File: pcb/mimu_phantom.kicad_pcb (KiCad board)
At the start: 2 copper layers, 50 x 27 mm, 35 parts, among them J1 OPT, SW1 SW_Push, SW2 SW_SPDT, U1 AQY211EH, U2 ATTINY88AU, U3 MCP16331CH, U4 H11F1M

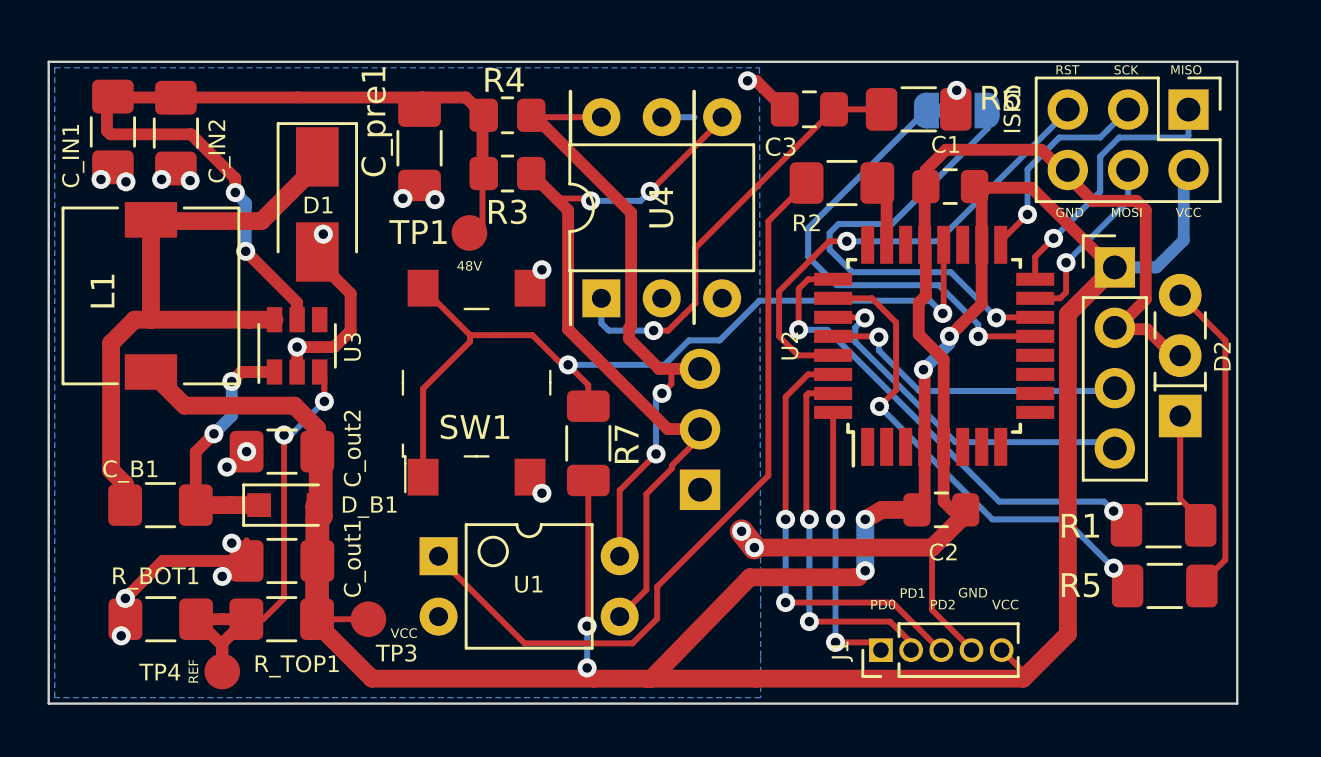
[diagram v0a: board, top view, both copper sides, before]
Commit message: First impression of new v3!
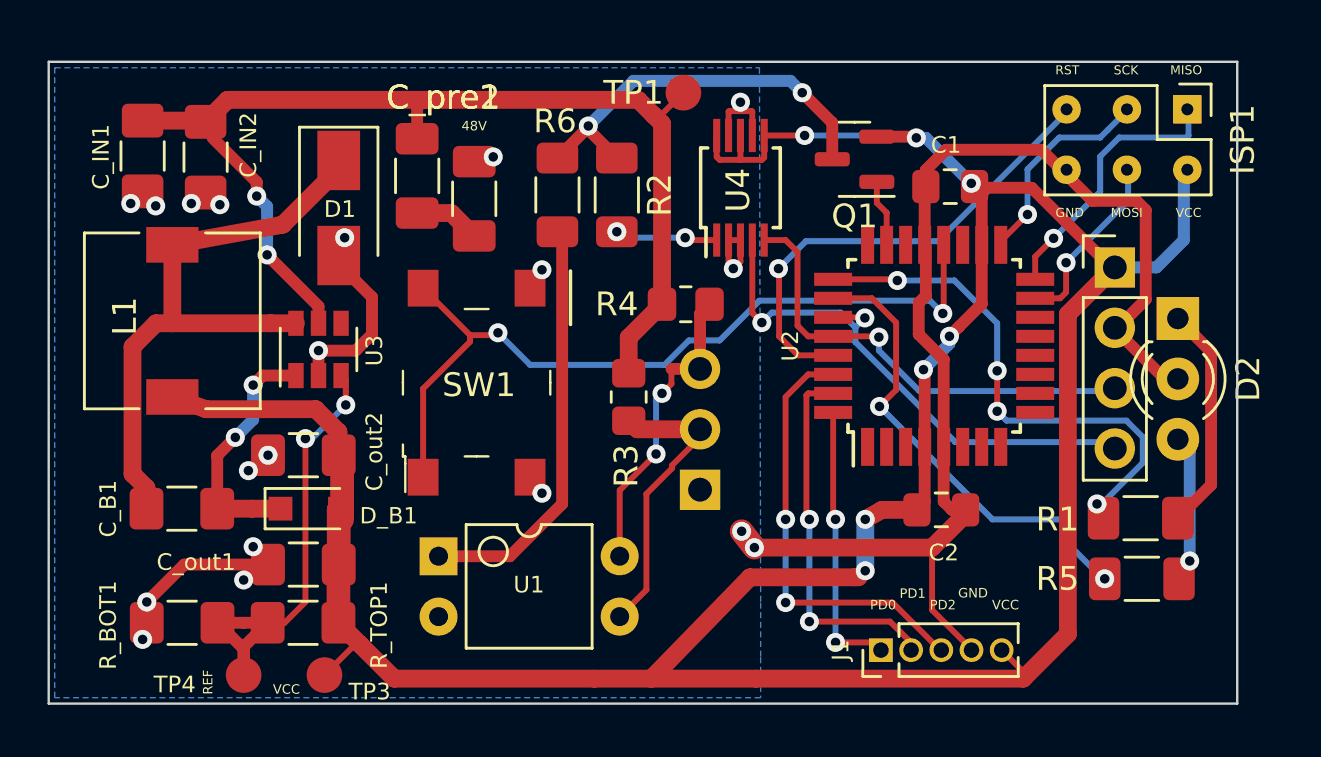
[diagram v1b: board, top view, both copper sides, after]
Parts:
- removed C3: 47nF, Capacitor_SMD:C_0805_2012Metric_Pad1.18x1.45mm_HandSolder
- removed R7: 1k, Capacitor_SMD:C_1206_3216Metric_Pad1.33x1.80mm_HandSolder
- removed SW2: SW_SPDT, Jumper:SolderJumper-3_P1.3mm_Bridged12_RoundedPad1.0x1.5mm_NumberLabels
- added C_pre2: 50-100uF @24V, Capacitor_SMD:C_1206_3216Metric_Pad1.33x1.80mm_HandSolder, F.Cu at (117.9, 78.8)
- added Q1: BSS84, Package_TO_SOT_SMD:SOT-23, F.Cu at (133.9, 77.1)
- C_pre1: value 100uF -> 50-100uF @24V
- D2: value LED_Dual_ACA -> LED_Dual_KAK; footprint LED_THT:LED_Rectangular_W5.0mm_H2.0mm-3Pins -> LED_THT:LED_D3.0mm-3
- ISP1: footprint Connector_PinHeader_2.54mm:PinHeader_2x03_P2.54mm_Vertical -> ProjectLibrary:PinHeader_2x03_P2.54mm_Vertical_pogo
- R2: value 1k -> 12R; footprint Resistor_SMD:R_1206_3216Metric_Pad1.42x1.75mm_HandSolder -> Resistor_SMD:R_1206_3216Metric_Pad1.30x1.75mm_HandSolder
- R6: value 100R -> 68R; footprint Capacitor_SMD:C_1206_3216Metric_Pad1.33x1.80mm_HandSolder -> Resistor_SMD:R_1206_3216Metric_Pad1.30x1.75mm_HandSolder
- U1: value AQY211EH -> PC817
- U4: value H11F1M -> AD5258; footprint Package_DIP:DIP-6_W7.62mm -> Package_SO:MSOP-10_3x3mm_P0.5mm
- moved R6 15.6 mm to (121.4, 78.6), turned to -90 degrees
- moved R4 10.9 mm to (126.8, 83.2)
- moved TP1 10.8 mm to (126.7, 74.3)
- moved R3 10.7 mm to (124.4, 87.1), turned to 90 degrees
- moved R2 9.48 mm to (123.9, 78.6), turned to 90 degrees
- moved U4 7.47 mm to (129.1, 78.3)
- moved D2 4.10 mm to (147.5, 83.8), turned to -90 degrees
- moved TP3 2.99 mm to (111.6, 98.8)
- moved C_IN1 1.61 mm to (104.0, 77.0)
- moved C_IN2 1.61 mm to (106.6, 77.0)
- moved L1 1.38 mm to (105.2, 83.9)
- moved C_pre1 1.17 mm to (115.5, 77.8)
- moved R1 1.01 mm to (145.9, 92.2)
- moved R5 1.01 mm to (146.0, 94.8)
- moved C_out1 0.91 mm to (110.7, 94.2)
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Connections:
- C_pre1 pad 2: XLR_GND -> Net-(C_pre1-Pad2)
- R2 pad 1: MUTE -> Net-(R2-Pad1)
- R2 pad 2: Net-(R2-Pad2) -> Net-(Q1-Pad3)
- R6 pad 1: ATT -> Net-(Q1-Pad3)
- R6 pad 2: Net-(C3-Pad1) -> Net-(U1-Pad1)
- U1 pad 1: Net-(R2-Pad2) -> Net-(U1-Pad1)
- U2 pad 1: Net-(U2-Pad1) -> unconnected-(U2-Pad1)
- U2 pad 10: Net-(U2-Pad10) -> unconnected-(U2-Pad10)
- U2 pad 11: Net-(U2-Pad11) -> unconnected-(U2-Pad11)
- U2 pad 12: Net-(U2-Pad12) -> unconnected-(U2-Pad12)
- U2 pad 13: OC1A -> unconnected-(U2-Pad13)
- U2 pad 14: OC1B -> unconnected-(U2-Pad14)
- U2 pad 19: Net-(U2-Pad19) -> unconnected-(U2-Pad19)
- U2 pad 2: Net-(U2-Pad2) -> unconnected-(U2-Pad2)
- U2 pad 22: Net-(U2-Pad22) -> unconnected-(U2-Pad22)
- U2 pad 23: MUTE -> MUTE_DRIVE
- U2 pad 24: Net-(U2-Pad24) -> unconnected-(U2-Pad24)
- U2 pad 3: Net-(U2-Pad3) -> unconnected-(U2-Pad3)
- U2 pad 6: Net-(U2-Pad6) -> unconnected-(U2-Pad6)
- U2 pad 7: Net-(U2-Pad7) -> unconnected-(U2-Pad7)
- U2 pad 8: Net-(U2-Pad8) -> unconnected-(U2-Pad8)
- U2 pad 9: Net-(U2-Pad9) -> unconnected-(U2-Pad9)
- U3 pad 4: Net-(U3-Pad4) -> unconnected-(U3-Pad4)
- U4 pad 1: Net-(C3-Pad1) -> Net-(R2-Pad1)
- U4 pad 3: (no net) -> XLR_GND
- U4 pad 4: XLR_HOT -> SDA
- U4 pad 5: (no net) -> SCL
- U4 pad 6: XLR_COLD -> VCC
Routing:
- net Net-(R2-Pad2): track 32.1 -> 0.00 mm
- net XLR_HOT: track 32.2 -> 12.3 mm, vias 2 -> 0
- net OC1B: track 19.8 -> 0.00 mm, vias 1 -> 0
- net OC1A: track 19.7 -> 0.00 mm, vias 1 -> 0
- net Net-(C3-Pad1): track 18.2 -> 0.00 mm, vias 1 -> 0
- net Net-(U1-Pad1): track 0.00 -> 17.6 mm
- net Net-(Q1-Pad3): track 0.00 -> 17.1 mm, vias 0 -> 2
- net XLR_COLD: track 26.0 -> 12.9 mm
- net +BATT: track 36.2 -> 46.8 mm
- net SDA: track 14.4 -> 22.4 mm, vias 1 -> 2
- net Net-(R5-Pad2): track 12.8 -> 5.33 mm, vias 0 -> 1
- net SCL: track 12.7 -> 19.1 mm
- net VCC: track 120.8 -> 127.0 mm, vias 6 -> 7
- net Net-(R1-Pad2): track 4.49 -> 9.56 mm
- net Net-(R2-Pad1): track 0.00 -> 4.34 mm, vias 0 -> 2
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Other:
- board text added: "MIMU Phantom v3 PP 12.22"
- board text removed: "MIMU Phantom v2 PP 10.21"
